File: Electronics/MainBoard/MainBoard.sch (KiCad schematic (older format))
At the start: 27 parts, among them J1 CONN_02X04, J2 DB9_Female, M1 Vibr_Motor, Q1 2N 2222A, Q2 2N 2222A, Q3 2N 2222A, Q4 2N 2222A, SW1 SW_PUSH, SW2 SPST, U1 ATMEGA168PA-AU

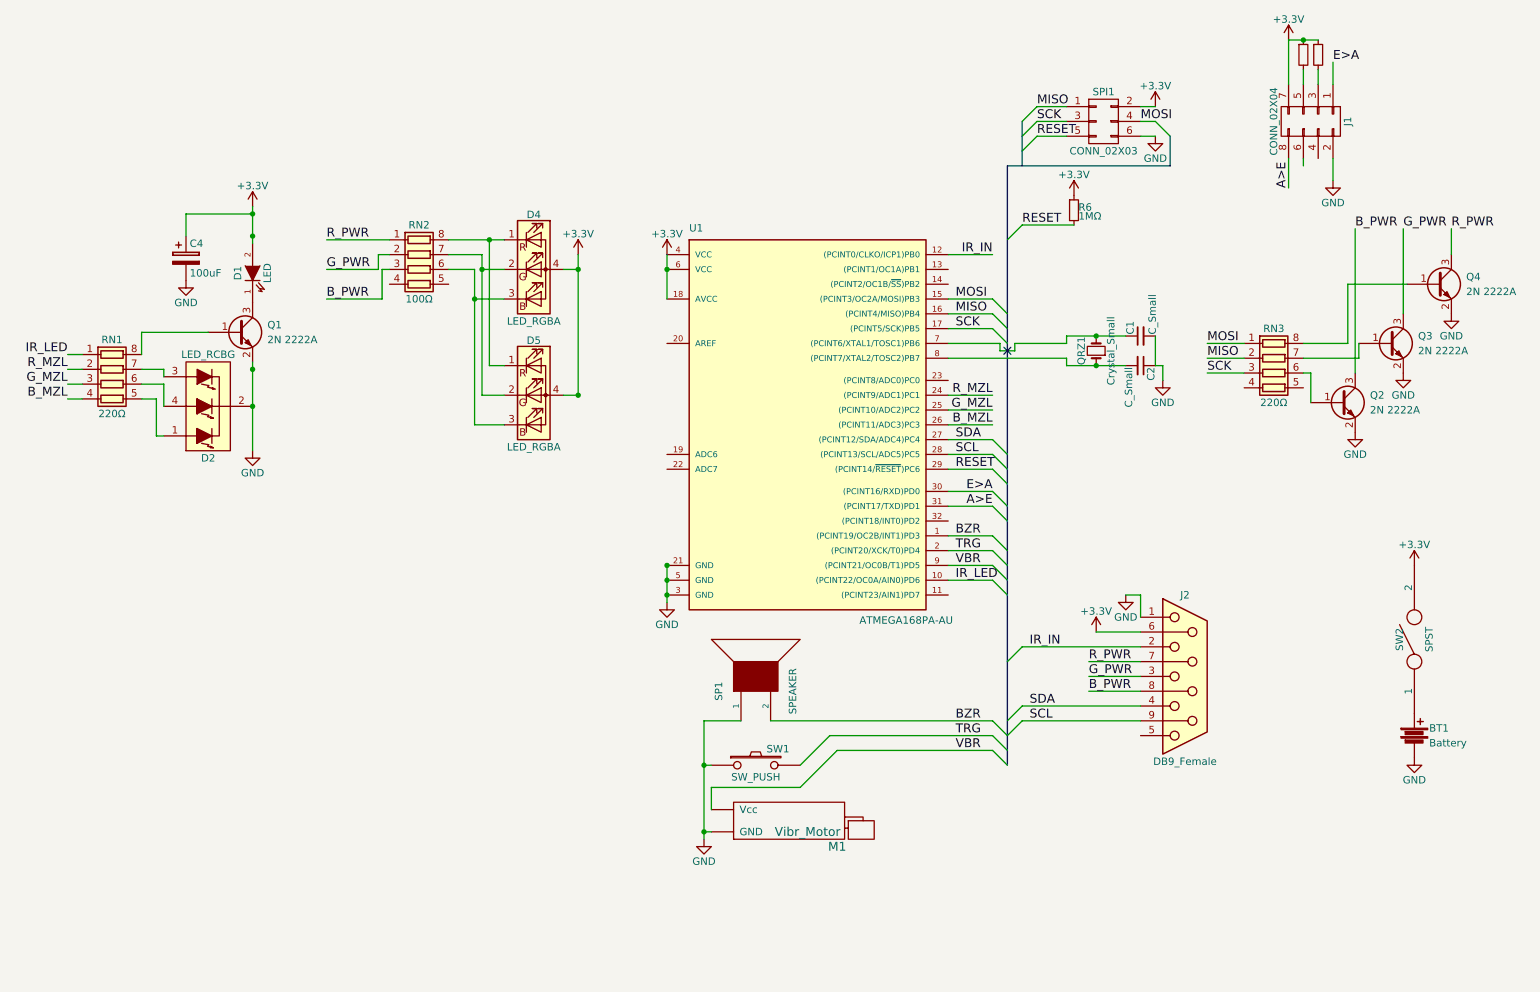
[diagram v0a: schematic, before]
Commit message: Final small changes
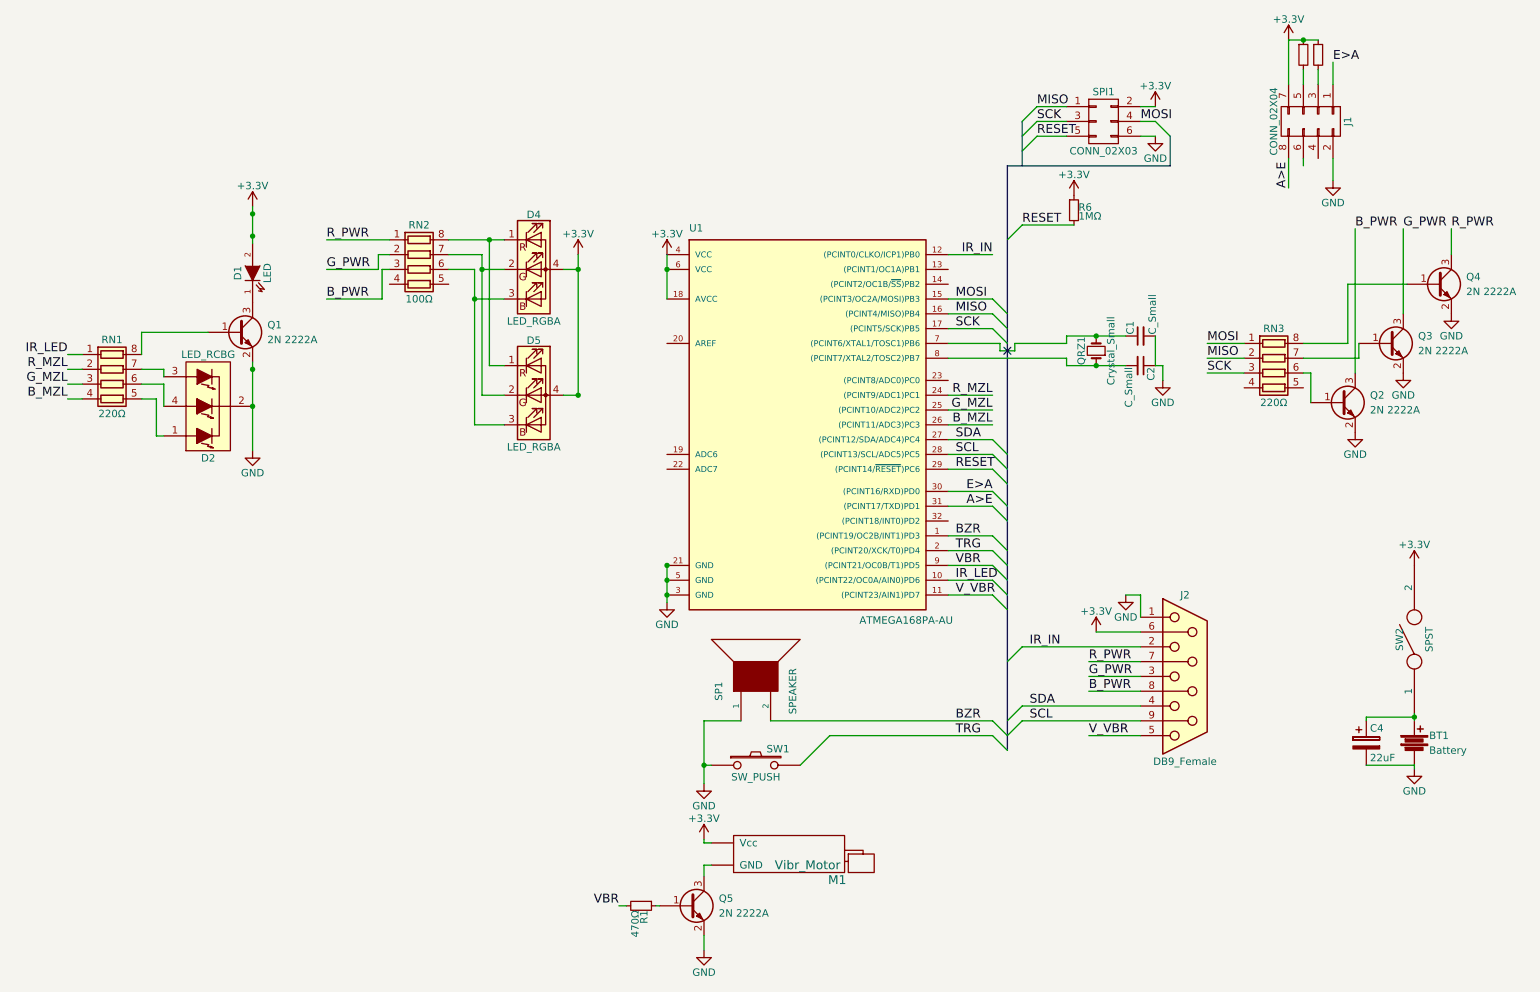
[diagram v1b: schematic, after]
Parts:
- added Q5: 2N 2222A, TO_SOT_Packages_SMD:SOT-23_Handsoldering, symbol Q_NPN_BEC
- added R1: 470Ω, Resistors_SMD:R_0603_HandSoldering, symbol R_Small
- C4: value 100uF -> 22uF; footprint Capacitors_SMD:CP_Elec_6.3x5.7 -> Capacitors_SMD:CP_Elec_5x5.3; URL https://www.reichelt.de/Elkos-SMD-Low-ESR-105-C/SMD-ELKO-10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 -> https://www.reichelt.de/Elkos-SMD-Low-ESR-105-C/SMD-ELKO-22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
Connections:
- net +3V3: now also M1.2 (Vcc); no longer C4.1
- net GND: now also Q5.2 (E); no longer M1.1 (GND)
- net VBR: now also R1.2; no longer M1.2 (Vcc)
- net at BT1.1, SW2.1: now also C4.1
- net V_VBR: now reaches U1.11 ((PCINT23/AIN1)PD7)
- net V_VBR: now also J2.5
- new net: M1.1 (GND), Q5.3 (C)
- new net: Q5.1 (B), R1.1
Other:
- moved on the sheet: BT1, C4, M1
